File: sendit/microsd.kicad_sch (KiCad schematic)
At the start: 10 parts, among them J9 Micro_SD_Card

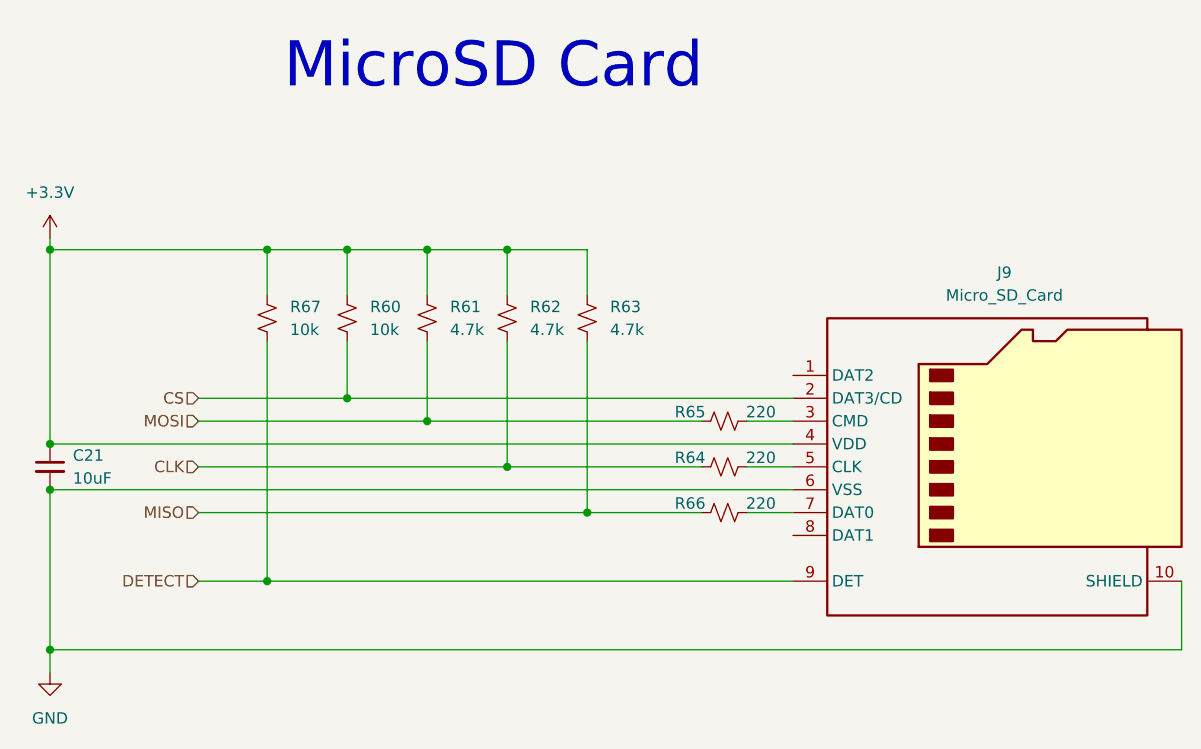
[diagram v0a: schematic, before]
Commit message: bigger update
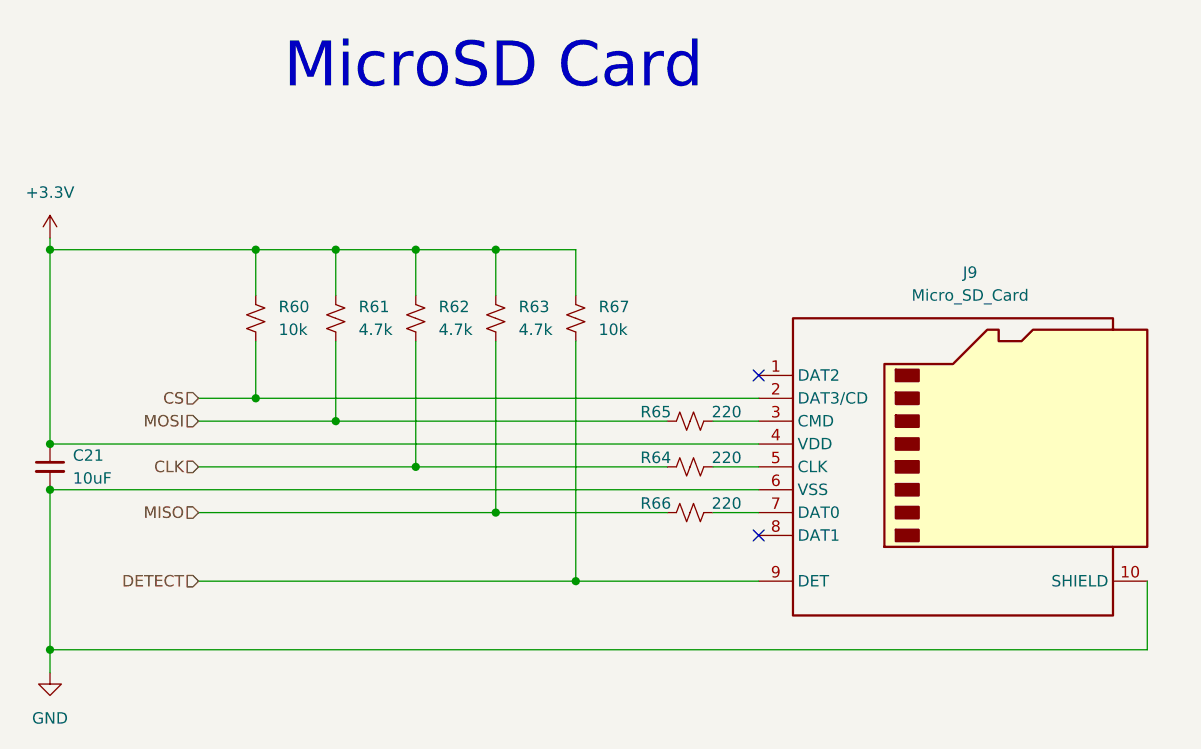
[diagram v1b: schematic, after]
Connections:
- no-connect marks 0 -> 2
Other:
- moved on the sheet: J9, R60, R61, R62, R63, R64, R65, R66, R67
